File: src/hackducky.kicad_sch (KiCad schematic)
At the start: 69 parts, among them J1 USB_A, J2 Conn_02x02_Top_Bottom, J3 Micro_SD_Card, J4 Conn_01x03_Pin, J6 Conn_01x04_Pin, P2 USB_C_Plug, SW3 BOOT_SEL, SW4 GP0, U2 AMS1117-3.3, U3 W25Q128JVS, U4 RP2040, U5 SRV05-4, U6 SRV05-4, Y1 Crystal_GND24

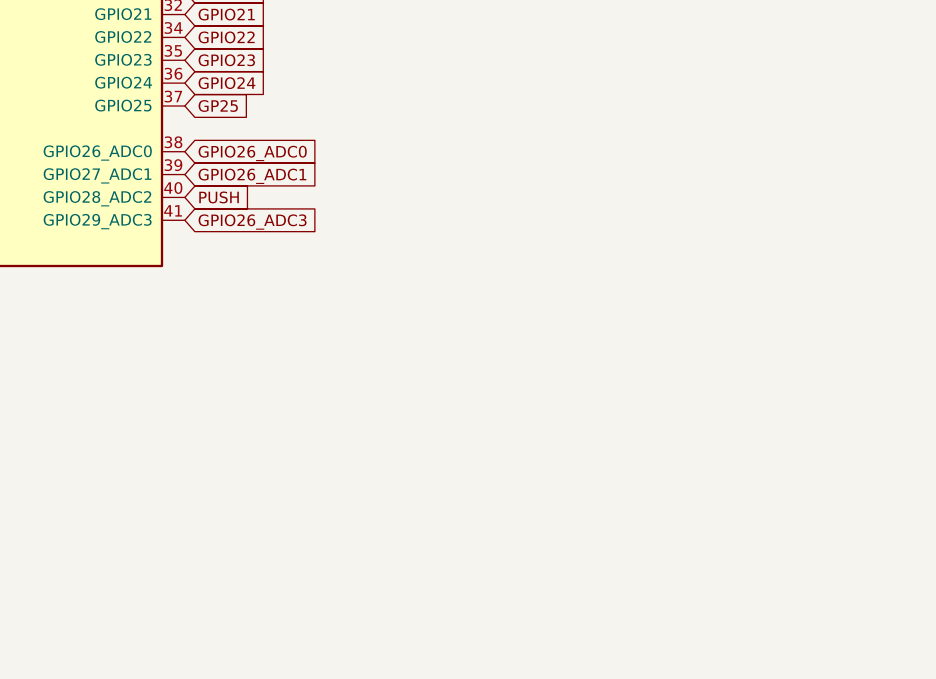
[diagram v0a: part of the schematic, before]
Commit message: final done with calip
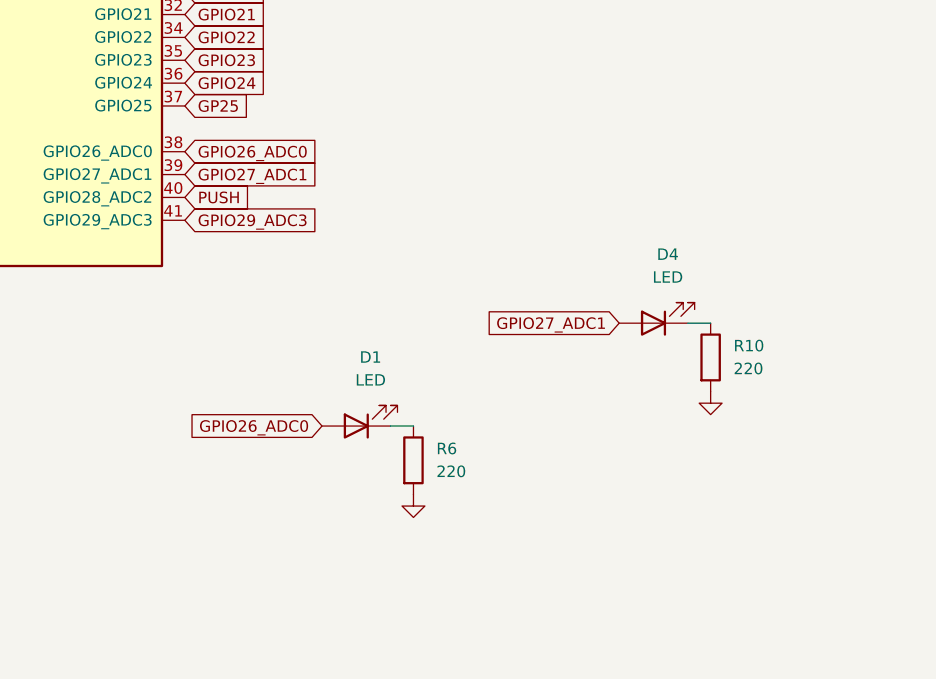
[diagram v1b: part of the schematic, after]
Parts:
- added D1, D4: LED, LED_SMD:LED_0402_1005Metric, symbol Device:LED
- added R10, R6: 220, Resistor_SMD:R_0402_1005Metric, symbol Device:R
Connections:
- net GND: now also R10.2, R6.2
- net GPIO26_ADC0: now also D1.2 (A)
- net GPIO26_ADC1: no longer U4.39 (GPIO27_ADC1)
- net GPIO26_ADC3: no longer U4.41 (GPIO29_ADC3)
- new net: D1.1 (K), R6.1
- new net: D4.1 (K), R10.1
- new net GPIO27_ADC1: D4.2 (A), U4.39 (GPIO27_ADC1)
- new net GPIO29_ADC3: U4.41 (GPIO29_ADC3)
